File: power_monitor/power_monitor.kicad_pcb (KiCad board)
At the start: 2 copper layers, 47.3 x 49.1 mm, 34 parts, among them J1 AVR-ISP-6, J2 Conn_01x06_Female, J3 Conn_01x04_Socket, J4 BATT, J5 VEH, U1 ATmega328-A, U2 ACS712ELCTR-20A, U4 AZ1117-3.3, U5 TS2940CW50, Y1 8M

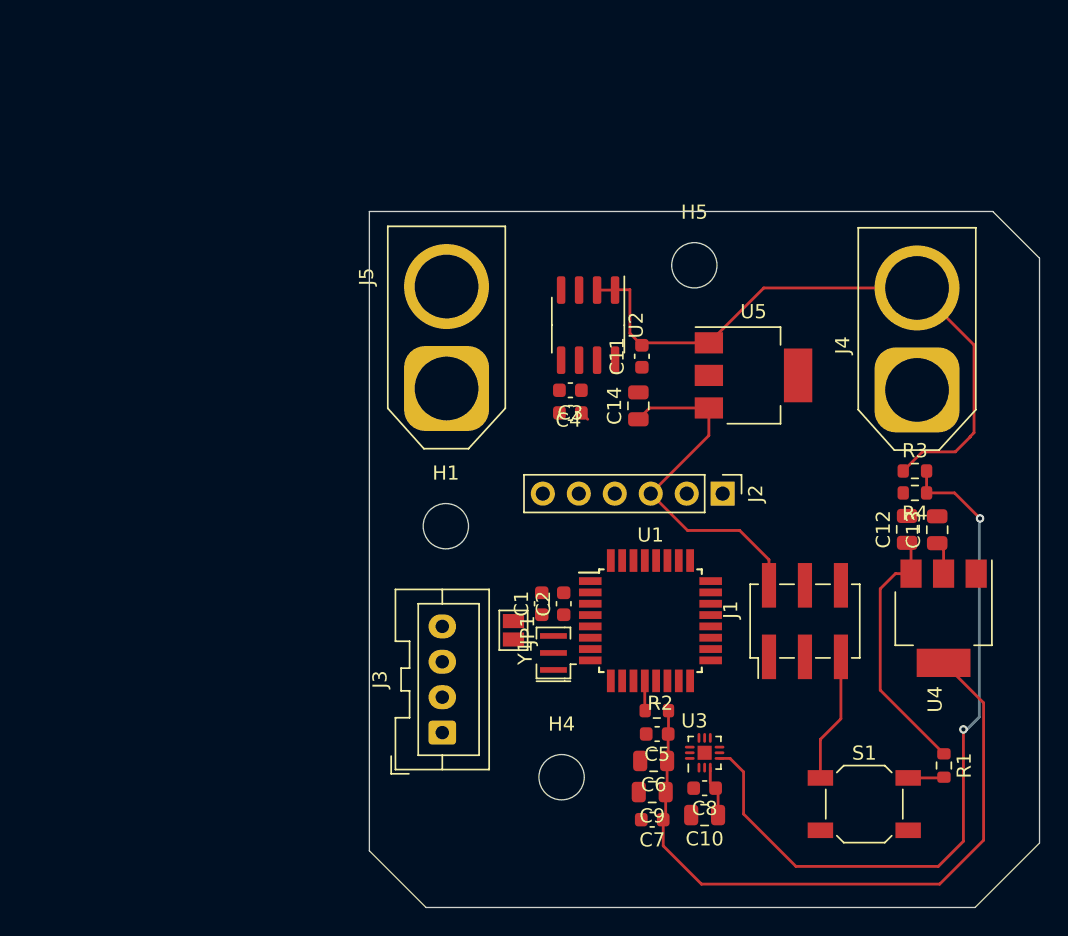
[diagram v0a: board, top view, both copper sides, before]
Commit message: PCB Layout finished
HAHAHAHAHA IT'S DONE. will commence routing.
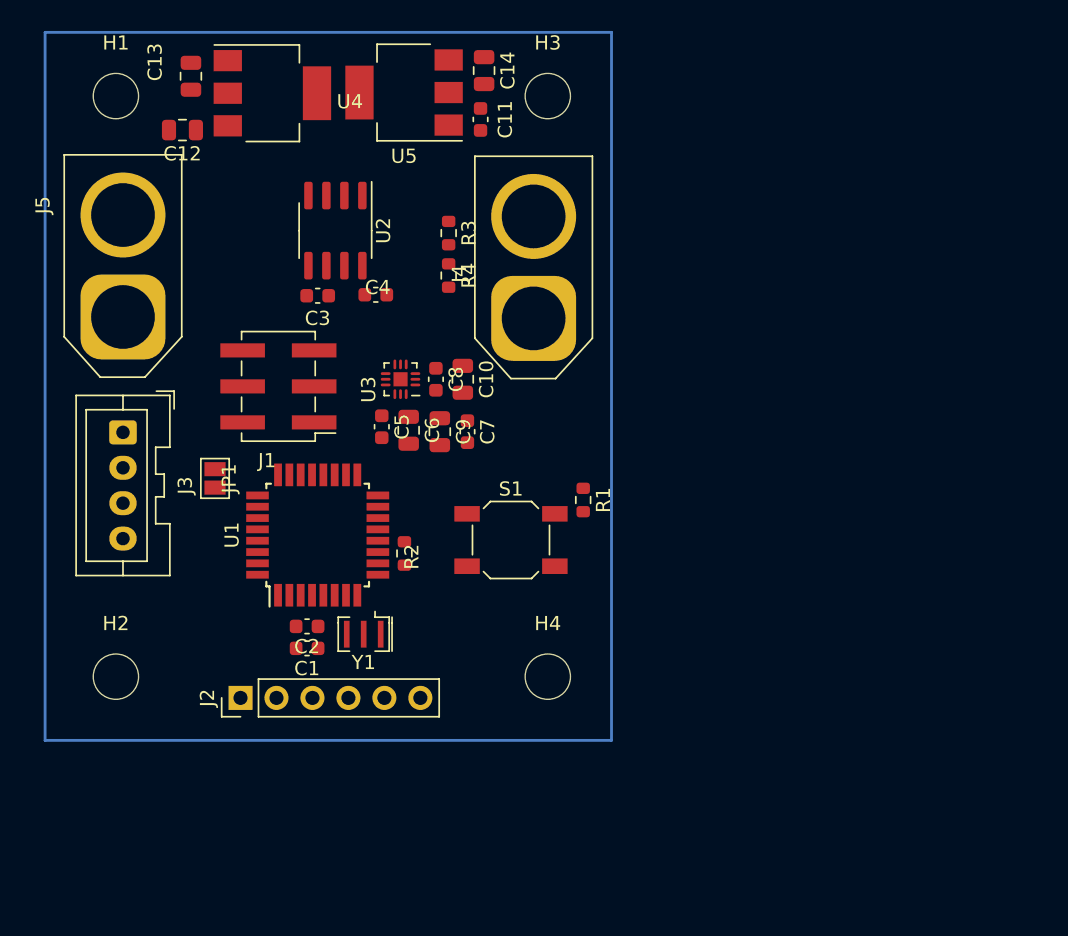
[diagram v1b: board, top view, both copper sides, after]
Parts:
- added H2: MountingHole, MountingHole:MountingHole_3.2mm_M3_ISO14580, F.Cu at (90.0, 81.0)
- moved C13 61.7 mm to (95.3, 38.6)
- moved U4 60.2 mm to (101.0, 39.8), turned to 0 degrees
- moved C12 58.4 mm to (94.7, 42.4), turned to 180 degrees
- moved J1 40.7 mm to (101.5, 60.5), turned to 180 degrees
- moved H1 38.3 mm to (90.0, 40.0)
- moved J2 37.0 mm to (98.8, 82.5), turned to 90 degrees
- moved R3 37.0 mm to (113.5, 49.7), turned to -90 degrees
- moved R4 36.3 mm to (113.5, 52.7), turned to -90 degrees
- moved C10 35.2 mm to (114.5, 60.0), turned to -90 degrees
- moved C8 34.6 mm to (112.6, 60.0), turned to -90 degrees
- moved U3 34.0 mm to (110.1, 60.0), turned to 180 degrees
- moved U5 31.7 mm to (110.3, 39.8), turned to 180 degrees
- moved R1 31.6 mm to (123.0, 68.5)
- moved S1 31.2 mm to (117.9, 71.3)
- moved J3 31.0 mm to (90.5, 63.8), turned to -90 degrees
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- renumbered H5 to H3
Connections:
- J1 pad 2: +5V -> +3V3
- J2 pad 3: +5V -> +3V3
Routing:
- net /BATT_DIVIDED: track 52.4 -> 0.00 mm, vias 2 -> 0
- net +3V3: track 51.6 -> 0.00 mm
- net +BATT: track 46.0 -> 0.00 mm
- net +5V: track 44.2 -> 0.00 mm
- net RESET: track 11.7 -> 0.00 mm
- net Net-(U3-REFIN+): track 3.58 -> 0.00 mm
- net CS: track 2.11 -> 0.00 mm
- net MISO: track 0.00 -> 1.08 mm
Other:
- board outline removed
